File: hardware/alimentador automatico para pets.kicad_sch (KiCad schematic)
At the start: 25 parts, among them J1 Conn_01x02, J2 Conn_01x04, J3 Conn_01x03, J4 Conn_01x03, J5 Conn_01x02, J6 Conn_01x05, J7 Conn_01x02, J8 Conn_01x04, SW1 SW_Push, SW2 SW_Push, SW3 SW_Push, U1 ESP32-DEVKIT-V1, U2 HX711_module

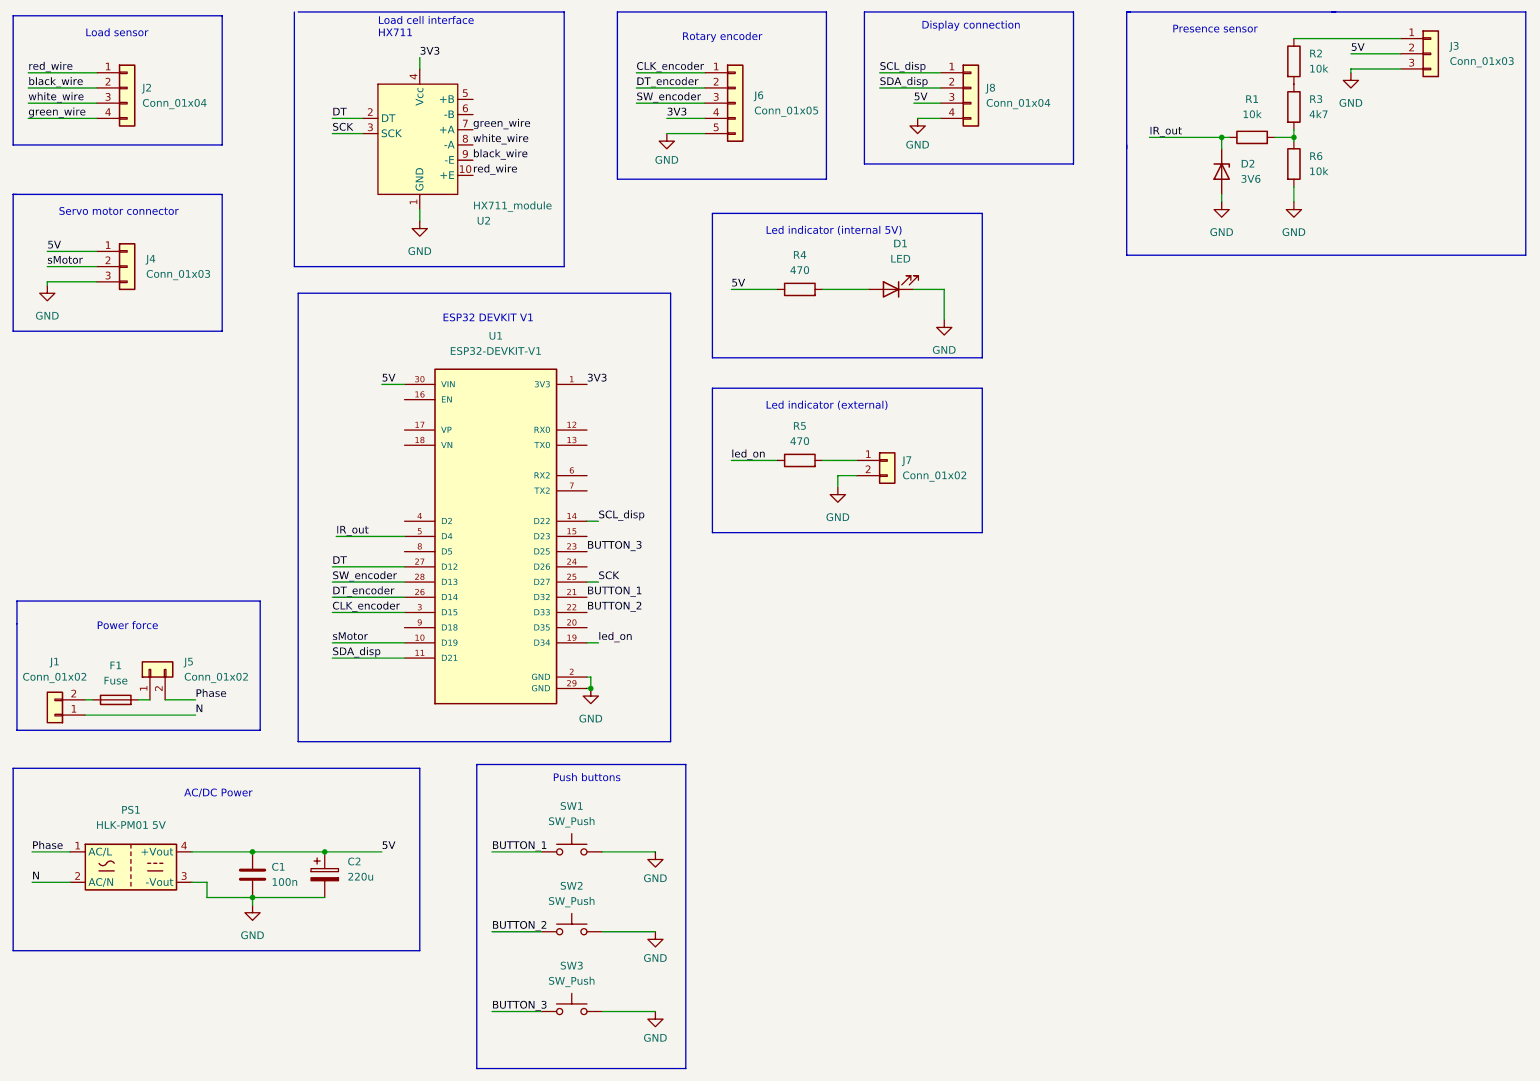
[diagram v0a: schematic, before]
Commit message: rearrange schematic
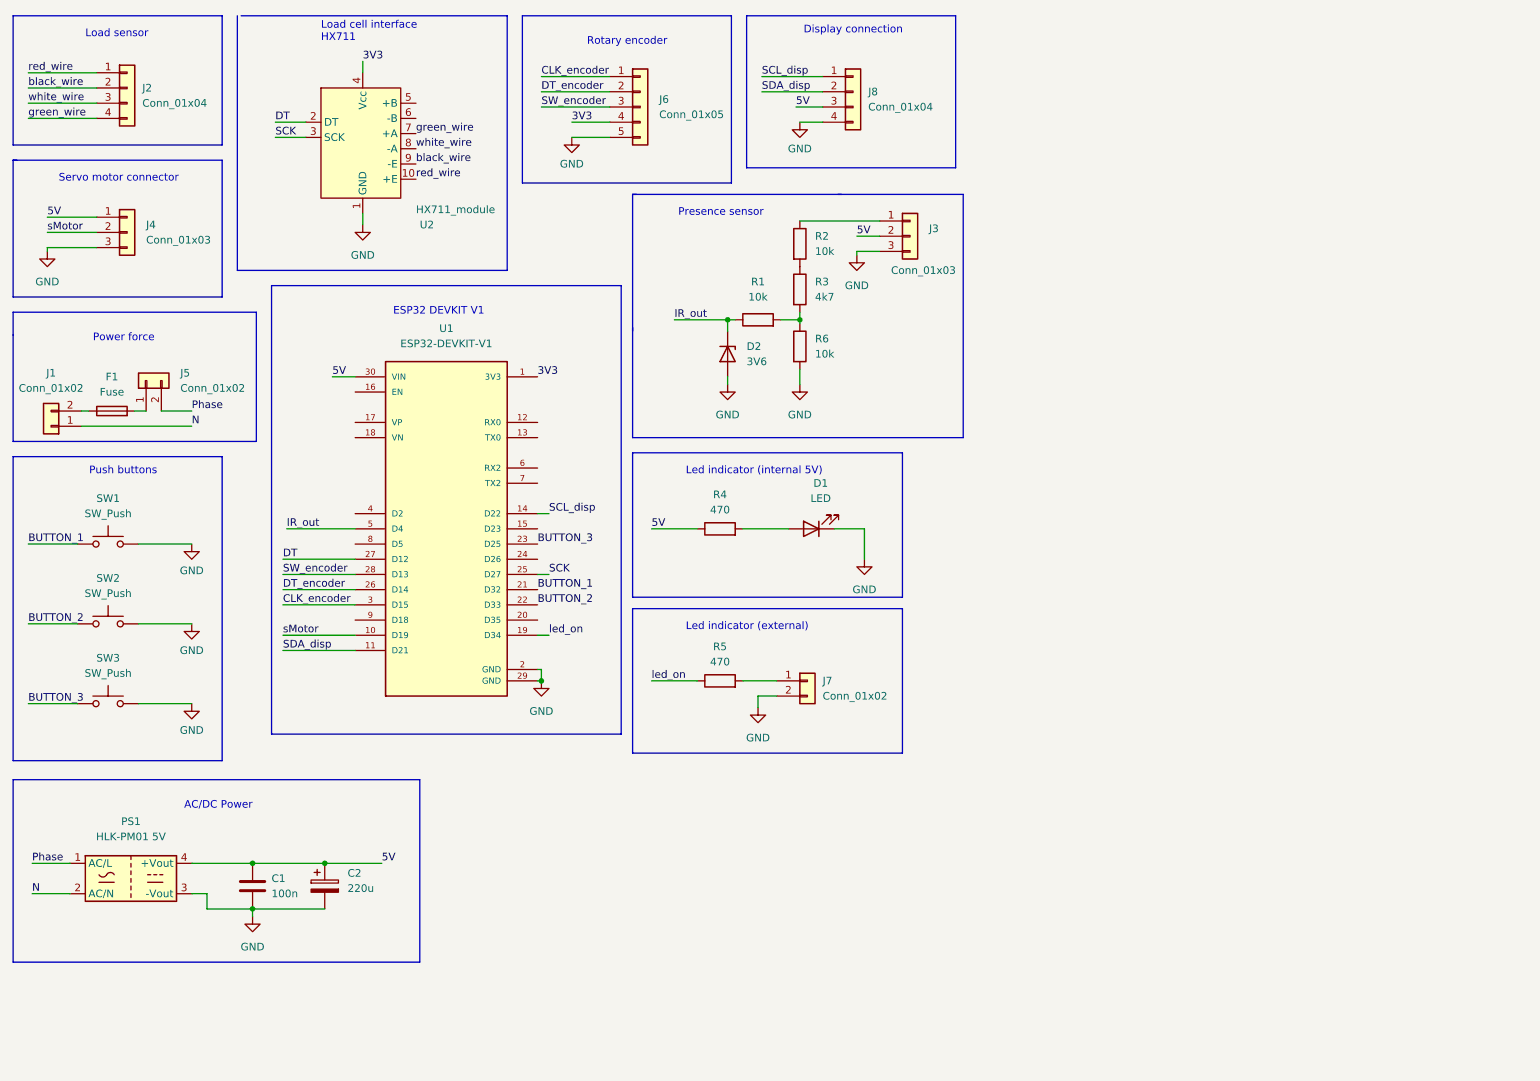
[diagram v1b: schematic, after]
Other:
- moved on the sheet: C1, C2, D1, D2, F1, J1, J3, J4, J5, J6, J7, J8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
